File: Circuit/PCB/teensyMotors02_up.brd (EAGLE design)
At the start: 76.3 x 157.6 mm, 66 parts, among them SW1 219-10, U1 MUX-74HC4067

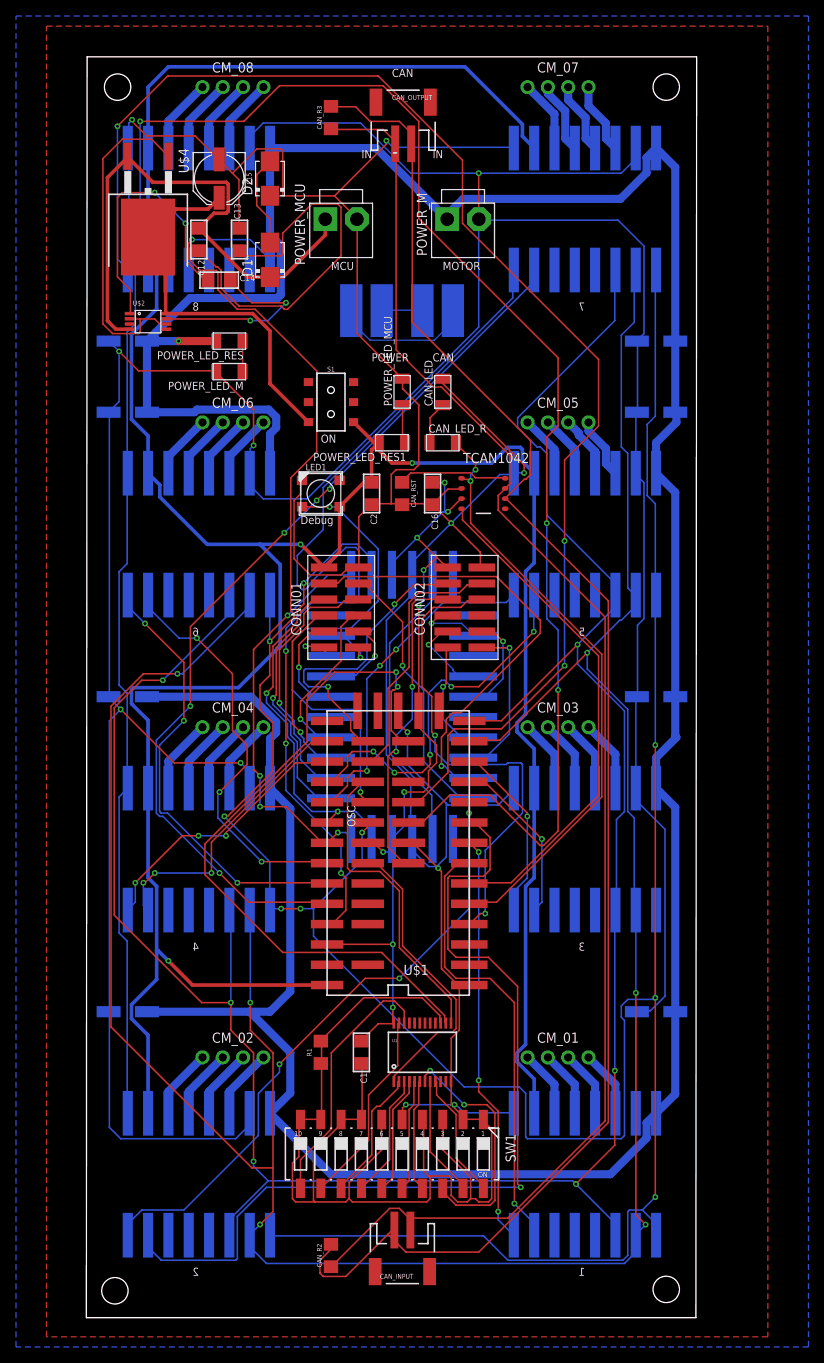
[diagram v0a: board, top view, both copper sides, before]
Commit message: circuit update
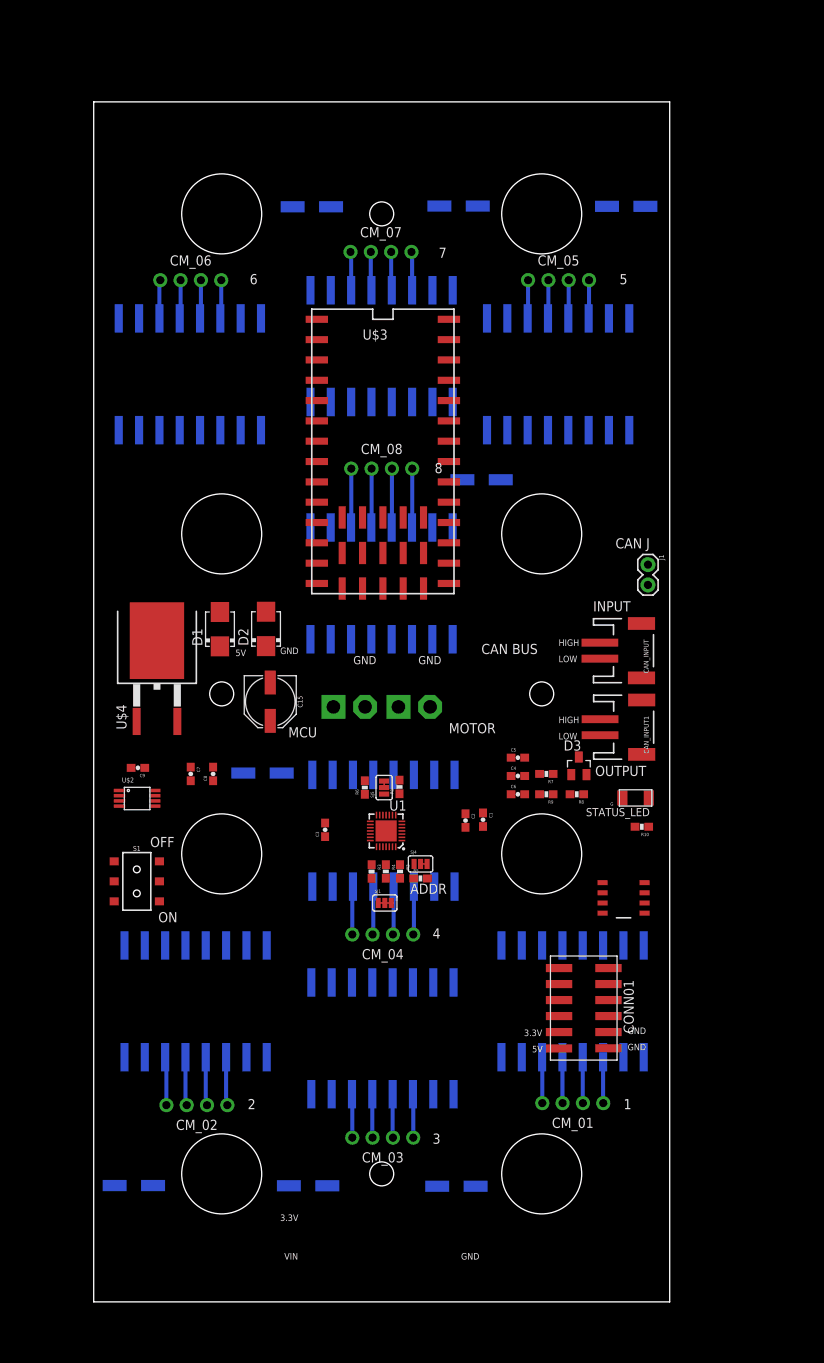
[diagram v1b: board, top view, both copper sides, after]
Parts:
- removed C10, C11: 100uF, SparkFun-Capacitors:PANASONIC_D
- removed C12, C13, C16: 0.1uf, microbuilder:1206
- removed C14: 2.2uF, microbuilder:1206
- removed CAN_LED, POWER_LED_M, POWER_LED_MCU: LEDFAB1206, fab:LED1206FAB
- removed CAN_LED_R, POWER_LED_RES, POWER_LED_RES1: 500, fab:R1206FAB
- removed CAN_OUTPUT: (no value), SparkFun-Connectors:JST-2-SMD
- removed CAN_R2, CAN_R3: 120ohm, SparkFun-Resistors:1206
- removed CAN_RST: 10K, SparkFun-Resistors:1206
- removed CONN02: TMMH-105-12, TMMH-105-XX-XX-DV:TMMH-105-12
- removed INPUT_POWER_1: MOLEX4015, MOLEX4015:MOLEX4015
- removed J2: (no value), SparkFun-Connectors:1X06_SMD_MALE
- removed J3, J4: (no value), SparkFun-Connectors:1X10_SMD_MALE
- removed LED1: (no value), SK6812:LED5050_N
- removed STANDOFF5, STANDOFF6, STANDOFF7, STANDOFF8: STAND-OFF, SparkFun-Electromechanical:STAND-OFF
- removed SW1: 219-10, switch-dil:CTS-219-10
- removed TCAN1042: Value, TCAN1042DRQ1:D0008A_N
- added C3: 0.1uF, SparkFun-Capacitors:0603-CAP
- added CAN_INPUT1: (no value), SparkFun-Connectors:JST-2-SMD
- added D3: PESD1CAN, diode:SOT23
- added MC1, MC2, MC3, MC4, MC5, MC6, MC7, MC8: 100uF, SparkFun-Capacitors:PANASONIC_D
- added R10: 500, SparkFun-Resistors:0603-RES
- added R2, R3, R4, R5, R6, R9: 10K, SparkFun-Resistors:0603-RES
- added R7, R8: 60, SparkFun-Resistors:0603-RES
- added SJ1: (no value), SparkFun-Passives:PAD-JUMPER-3-3OF3_NC_BY_TRACE_YES_SILK_FULL_BOX
- added SJ4, SJ5: (no value), SparkFun-Passives:PAD-JUMPER-3-2OF3_NC_BY_TRACE_YES_SILK_FULL_BOX
- added STATUS_LED: LEDFAB1206, fab:LED1206FAB
- added U$3: TEENSY_4.0_WITH_SMD_HEADER_PINSTEENSY_4.0_SMD, Teensy4:TEENSY_4.0_SMD
- C1, C2: value 0.1uf -> 0.1uF; device microbuilder:1206 -> SparkFun-Capacitors:0603-CAP
- C4, C9: value 100uF -> 2.2uf; device SparkFun-Capacitors:PANASONIC_D -> SparkFun-Capacitors:0603-CAP
- C5: value 100uF -> 4.7uf; device SparkFun-Capacitors:PANASONIC_D -> SparkFun-Capacitors:0603-CAP
- C6, C7, C8: value 100uF -> 0.1uf; device SparkFun-Capacitors:PANASONIC_D -> SparkFun-Capacitors:0603-CAP
- CM_01, CM_02, CM_03, CM_04, CM_05, CM_06, CM_07, CM_08: value 1X04_SMD_STRAIGHT_COMBO -> 1X04_STRAIGHT
- J1: device SparkFun-Connectors:1X06_SMD_MALE -> SparkFun-Connectors:1X02
- R1: value (none) -> 10K; device SparkFun-Resistors:1206 -> SparkFun-Resistors:0603-RES
- U$1: value TEENSY_3.1-3.2_ALL_PINS&PADS_SMD -> SN65HVD232Q; device Teensy_3_and_LC_Series_Boards_v1.4:TEENSY_3.0-3.2_ALL_PINS_&_PADS_SMD -> TCAN1042DRQ1:SN65HVD232Q
- U1: value MUX-74HC4067 -> SX1509; device SparkFun:SSOP24 -> SparkFun-DigitalIC:QFN-28
- moved CAN_INPUT 81.2 mm to (69.1, 84.5), turned to 270 degrees
- moved C8 71.5 mm to (17.0, 69.1), flipped to the top, turned to 90 degrees
- moved C15 65.7 mm to (24.2, 78.1)
- moved S1 64.6 mm to (7.48, 55.7)
- moved POWER_M 61.3 mm to (42.2, 77.5), flipped to the bottom, turned to 180 degrees
- moved POWER_MCU 61.0 mm to (34.0, 77.5), flipped to the bottom, turned to 180 degrees
- moved U$2 59.6 mm to (7.52, 66.1)
- moved CONN01 59.0 mm to (63.3, 39.6), turned to 270 degrees
- moved C7 59.0 mm to (14.2, 69.1), flipped to the top, turned to 270 degrees
- moved C5 58.2 mm to (55.1, 71.1), flipped to the top, turned to 0 degrees
- moved D2 56.3 mm to (23.6, 87.2)
- moved CM_03 55.8 mm to (38.2, 23.6), turned to 180 degrees
- moved U$4 52.4 mm to (10.0, 84.8), turned to 0 degrees
- moved MOTOR_08 52.1 mm to (38.1, 92.9)
- moved CM_08 51.2 mm to (38.1, 107.2)
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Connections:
- net MUS_S1 renamed OSCIO_SX0
- removed net AGND: U$1.AGND
- removed net AREF: U$1.AREF
- removed net C0: SW1.20, U1.9
- removed net C1: SW1.19, U1.8
- removed net C2: SW1.18, U1.7
- removed net C3: SW1.17, U1.6
- removed net C4: SW1.16, U1.5
- removed net C5: SW1.15, U1.4
- removed net C6: SW1.14, U1.3
- removed net C7: SW1.13, U1.2
- removed net C8: SW1.12, U1.23
- removed net C9: SW1.11, U1.22
- removed net CAN_RX: TCAN1042.4, U$1.4
- removed net CAN_TX: CAN_LED_R.2, TCAN1042.1, U$1.3
- removed net GND_IN: INPUT_POWER_1.GND_01, INPUT_POWER_1.GND_02
- removed net I2CM_0: CONN01.1, J3.9
- removed net I2CM_1: CONN01.2, J3.8
- removed net I2CM_10: CONN02.1, J4.3
- removed net I2CM_11: CONN02.2, J4.4
- removed net I2CM_12: CONN02.3, J4.6
- removed net I2CM_13: CONN02.4, J4.7
- removed net I2CM_14: J4.8
- removed net I2CM_15: CONN02.6, J4.9
- removed net I2CM_2: CONN01.3, J3.7
- removed net I2CM_3: CONN01.4, J3.6
- removed net I2CM_4: CONN01.5, J3.4
- removed net I2CM_5: CONN01.6, J3.3
- removed net I2CM_6: CONN01.7, J3.2
- removed net I2CM_7: CONN01.8, J3.1
- removed net I2CM_8: CONN01.9, J4.1
- removed net I2CM_9: CONN01.10, J4.2
- removed net IC2M_14: CONN02.5
- removed net LED_DEBUG: LED1.4-DIN, U$1.32
- removed net MENABLE: MOTOR_01.ENA, MOTOR_02.ENA, MOTOR_03.ENA, MOTOR_04.ENA, MOTOR_05.ENA, MOTOR_06.ENA, MOTOR_07.ENA, MOTOR_08.ENA, U$1.33
- removed net MUX_INT: J1.1
- removed net MUX_OSCIO: J2.1
- removed net MUX_RESET: J1.2, J2.2
- removed net MUX_S0: U$1.26
- removed net MUX_S1: U$1.27
- removed net MUX_S2: U$1.28, U1.14
- removed net MUX_S3: U$1.31, U1.13
- removed net MUX_SCL: J1.6, J2.6, U$1.19/A5
- removed net MUX_SDA: J1.5, J2.5, U$1.18/A4
- removed net MUX_SIG: U$1.A13, U1.1
- removed net MUX_SO: U1.10
- removed net N$11: U$1.13
- removed net S_SCL: CONN02.10, U$1.29
- removed net S_SDA: CONN02.9, U$1.30
- removed net S_SEN_01: CONN02.8, U$1.A12
- removed net VCC1: J3.5
- removed net VCC2: J4.5
- removed net VCC_IN: INPUT_POWER_1.VCC_01, INPUT_POWER_1.VCC_02
- removed net VUSB: U$1.VUSB
- new net !INT_SX0: R1.1, U$3.13, U1.9
- new net !RESET_SX0: R3.1, U1.23
- new net 0_SX0: MOTOR_01.ENA, U1.27
- new net 10_SX0: MOTOR_06.ENA, U1.15
- new net 11_SX0: MOTOR_06.STBY, U1.16
- new net 12_SX0: MOTOR_07.ENA, U1.19
- new net 13_SX0: MOTOR_07.STBY, U1.20
- new net 14_SX0: MOTOR_08.ENA, U1.21
- new net 15_SX0: MOTOR_08.STBY, U1.22
- new net 1_SX0: MOTOR_01.STBY, U1.28
- new net 2_SX0: MOTOR_02.ENA, U1.1
- new net 3_SX0: MOTOR_02.STBY, U1.2
- new net 4_SX0: MOTOR_03.ENA, U1.5
- new net 5_SX0: MOTOR_03.STBY, U1.6
- new net 6_SX0: MOTOR_04.ENA, U1.7
- new net 7_SX0: MOTOR_04.STBY, U1.8
- new net 8_SX0: MOTOR_05.ENA, U1.13
- new net 9_SX0: MOTOR_05.STBY, U1.14
- new net ADDR0_SX0: SJ4.2, U1.26
- new net ADDR1_SX0: SJ5.2, U1.10
- new net CAN_RX2: CONN01.7, U$3.0
- new net CAN_RX3: U$1.R, U$3.30
- new net CAN_TX2: CONN01.8, U$3.1
- new net CAN_TX3: U$1.D, U$3.31
- new net N$10: R6.1, SJ5.1
- new net N$14: J1.1, R8.1
- new net N$8: R5.1, SJ4.1
- new net PIN_2: CONN01.6, U$3.2
- new net SCL_00: R2.1, U$3.19/A5, U1.25
- new net SCL_01: CONN01.1, U$3.16/A2
- new net SCL_02: CONN01.3, U$3.24
- new net SDA_00: R4.1, U$3.18/A4, U1.24
- new net SDA_01: CONN01.2, U$3.17/A3
- new net SDA_02: CONN01.4, U$3.25
- new net STATUS_PIN: R10.2, U$3.4
- new net TRQ1: MOTOR_01.1, MOTOR_02.1, MOTOR_03.1, MOTOR_04.1, MOTOR_05.1, MOTOR_06.1, MOTOR_07.1, MOTOR_08.1, U$3.32
- new net TRQ2: MOTOR_01.2, MOTOR_02.2, MOTOR_03.2, MOTOR_04.2, MOTOR_05.2, MOTOR_06.2, MOTOR_07.2, MOTOR_08.2, U$3.33
- net 3.3V: now also C2.1, C3.1, C4.1, C6.1, CONN01.9, R1.2, R3.2, R5.2, R6.2, SJ1.2, U$1.VCC, U$3.3.3V, U$3.3.3V1, U1.12, U1.18, U1.4; no longer C16.1, CONN02.11, J1.4, J2.4, TCAN1042.3, U$1.3.3V, U$1.3.3V1, U$1.3.3V2, U1.24
- net CAN_H: now also CAN_INPUT1.1, D3.1, R7.2, U$1.CANH; no longer CAN_OUTPUT.1, CAN_R2.1, CAN_R3.1, TCAN1042.7
- net CAN_L: now also CAN_INPUT1.2, D3.2, J1.2, U$1.CANL; no longer CAN_OUTPUT.2, CAN_R2.2, CAN_R3.2, TCAN1042.6
- net GND_M: now also MC1.-, MC2.-, MC3.-, MC4.-, MC5.-, MC6.-, MC7.-, MC8.-; no longer C10.-, C11.-, C4.-, C5.-, C6.-, C7.-, C8.-, C9.-, POWER_LED_M.2
- net GND_MCU: now also C3.2, C4.2, C5.2, C6.2, C8.2, CONN01.10, D3.3, R9.2, SJ4.3, SJ5.3, STATUS_LED.2, U$3.GND, U$3.GND1, U$3.GND2, U1.17, U1.29, U1.3; no longer C13.2, C16.2, CAN_LED.2, CAN_RST.2, CONN02.12, J1.3, J2.3, LED1.3-GND, POWER_LED_MCU.2, R1.1, R1.2, SW1.1, SW1.10, SW1.2, SW1.3, SW1.4, SW1.5, SW1.6, SW1.7, SW1.8, SW1.9, TCAN1042.2, U$1.GND1, U$1.GND2, U1.12, U1.15
- net MDIR_01: now also U$3.6; no longer U$1.6
- net MDIR_02: now also U$3.8; no longer U$1.8
- net MDIR_03: now also U$3.10; no longer U$1.10
- net MDIR_04: now also U$3.12; no longer U$1.15/A1
- net MDIR_05: now also U$3.15/A1; no longer U$1.17/A3
- net MDIR_06: now also U$3.21/A7; no longer U$1.21/A7
- net MDIR_07: now also U$3.23/A9; no longer U$1.23/A9
- net MDIR_08: now also U$3.27; no longer U$1.25
- net MMS1: now also U$3.28; no longer U$1.11
- net MMS2: now also U$3.29; no longer U$1.12
- net MSTEP_01: now also U$3.5; no longer U$1.5
- net MSTEP_02: now also U$3.7; no longer U$1.7
- net MSTEP_03: now also U$3.9; no longer U$1.9
- net MSTEP_04: now also U$3.11; no longer U$1.14/A0
- net MSTEP_05: now also U$3.14/A0; no longer U$1.16/A2
- net MSTEP_06: now also U$3.20/A6; no longer U$1.20/A6
- net MSTEP_07: now also U$3.22/A8; no longer U$1.22/A8
- net MSTEP_08: now also U$3.26; no longer U$1.24
- net N$1: now also R2.2, SJ1.3; no longer POWER_LED_M.1, POWER_LED_RES.1
- net N$13: now also C5.1, R7.1, R8.2; no longer LED1.2-DOUT
- net N$193: now also R10.1, STATUS_LED.1; no longer CAN_LED.1, CAN_LED_R.1
- net N$2: now also C9.1; no longer C14.2
- net N$3: now also U$1.VREF; no longer TCAN1042.5
- net N$5: now also C9.2; no longer C14.1
- net N$6: now also R9.1, U$1.RS; no longer CAN_RST.1, TCAN1042.8
- net N$7: now also R4.2, SJ1.1; no longer POWER_LED_MCU.1, POWER_LED_RES1.1
- net N$9: now also C7.2, C8.1; no longer C12.2, C13.1
- net NEO_PIXEL: now also CONN01.5, U$3.3; no longer CONN02.7, U$1.2
- net VBAT: now also U$3.VBAT; no longer U$1.VBAT
- net VCC_5V: now also S1.2, U$3.VIN; no longer C2.1, LED1.1-VDD, POWER_LED_RES1.2, S1.3, U$1.VIN
- net VCC_M: now also MC1.+, MC2.+, MC3.+, MC4.+, MC5.+, MC6.+, MC7.+, MC8.+; no longer C10.+, C11.+, C4.+, C5.+, C6.+, C7.+, C8.+, C9.+, POWER_LED_RES.2
- net VCC_MCU: now also C7.1; no longer C12.1
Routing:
- net GND_MCU: track 599.1 -> 0.00 mm, vias 8 -> 0
- net GND_M: track 420.2 -> 0.00 mm, vias 5 -> 0
- net VCC_M: track 406.5 -> 0.00 mm, vias 1 -> 0
- net MENABLE: track 404.0 -> 0.00 mm, vias 9 -> 0
- net VCC_5V: track 377.9 -> 0.00 mm, vias 3 -> 0
- net MMS1: track 335.7 -> 0.00 mm, vias 6 -> 0
- net MMS2: track 307.5 -> 0.00 mm, vias 6 -> 0
- net CAN_L: track 199.4 -> 0.00 mm
- net CAN_H: track 190.0 -> 0.00 mm
- net MSTEP_08: track 178.1 -> 0.00 mm, vias 3 -> 0
- net MDIR_08: track 169.9 -> 0.00 mm, vias 3 -> 0
- net MDIR_07: track 119.1 -> 0.00 mm, vias 3 -> 0
- net MSTEP_07: track 113.7 -> 0.00 mm, vias 5 -> 0
- net MSTEP_02: track 113.5 -> 0.00 mm, vias 1 -> 0
- net 3.3V: track 106.5 -> 0.00 mm, vias 9 -> 0
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- removed copper zone on layer 1, net GND_MCU
- removed copper zone on layer 16, net GND_MCU
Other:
- board size 76.3 x 157.6 mm -> 72 x 150 mm
- board text added: "5V"
- board text added: "ADDR"
- board text added: "CAN BUS"
- board text added: "CAN J"
- board text added: "G"
- board text added: "HIGH"
- board text added: "INPUT"
- board text added: "LOW"
- board text added: "OFF"
- board text added: "OUTPUT"
- board text added: "VIN"
- board text removed: "!INT"
- board text removed: "!RST"
- board text removed: "-"
- board text removed: "0"
- board text removed: "10"
- board text removed: "11"
- board text removed: "12"
- board text removed: "13"
- board text removed: "14"
- board text removed: "15"
- board text removed: "3V3"
- board text removed: "9"
- board text removed: "CAN"
- board text removed: "Debug"
- board text removed: "IN"
- board text removed: "OSC"
- board text removed: "POWER"
- board text removed: "SCL"
- board text removed: "SDA"
- board text removed: "VC1"
- board text removed: "VC2"
